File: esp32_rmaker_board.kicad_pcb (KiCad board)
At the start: 2 copper layers, 32 parts, among them Q1 BC817, Q2 BC817, Q3 BC817, Q4 BC817, Q5 BC817, Q6 BC817, U1 ESP32-DevKitC-MCU_Espressif, U10 DHT22, U2 DG142V-5.08-4, U3 DG142V-5.08-4, U4 DG142V-5.08-4, U5 DG142V-5.08-4, U6 LM1117-5.0, U7 DG142V-5.08-4, U9 OPA340NA

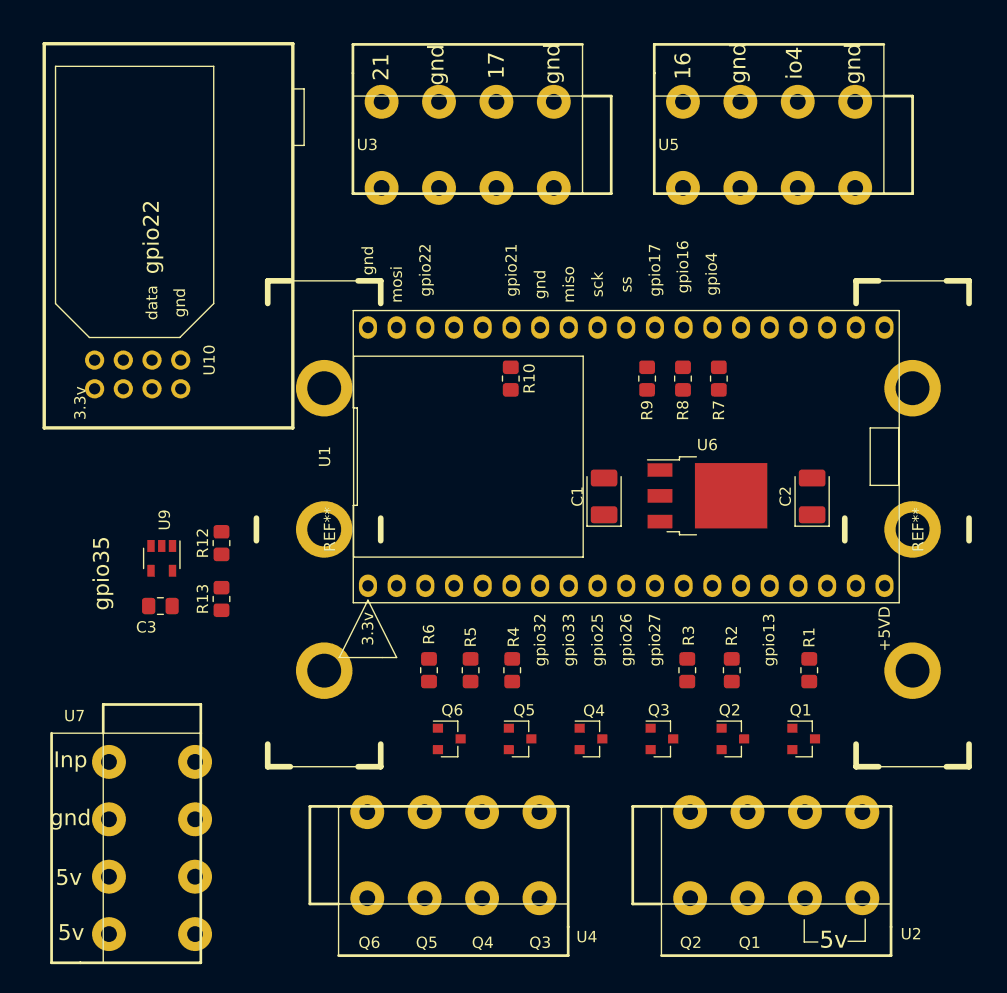
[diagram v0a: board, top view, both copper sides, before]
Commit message: v1.0
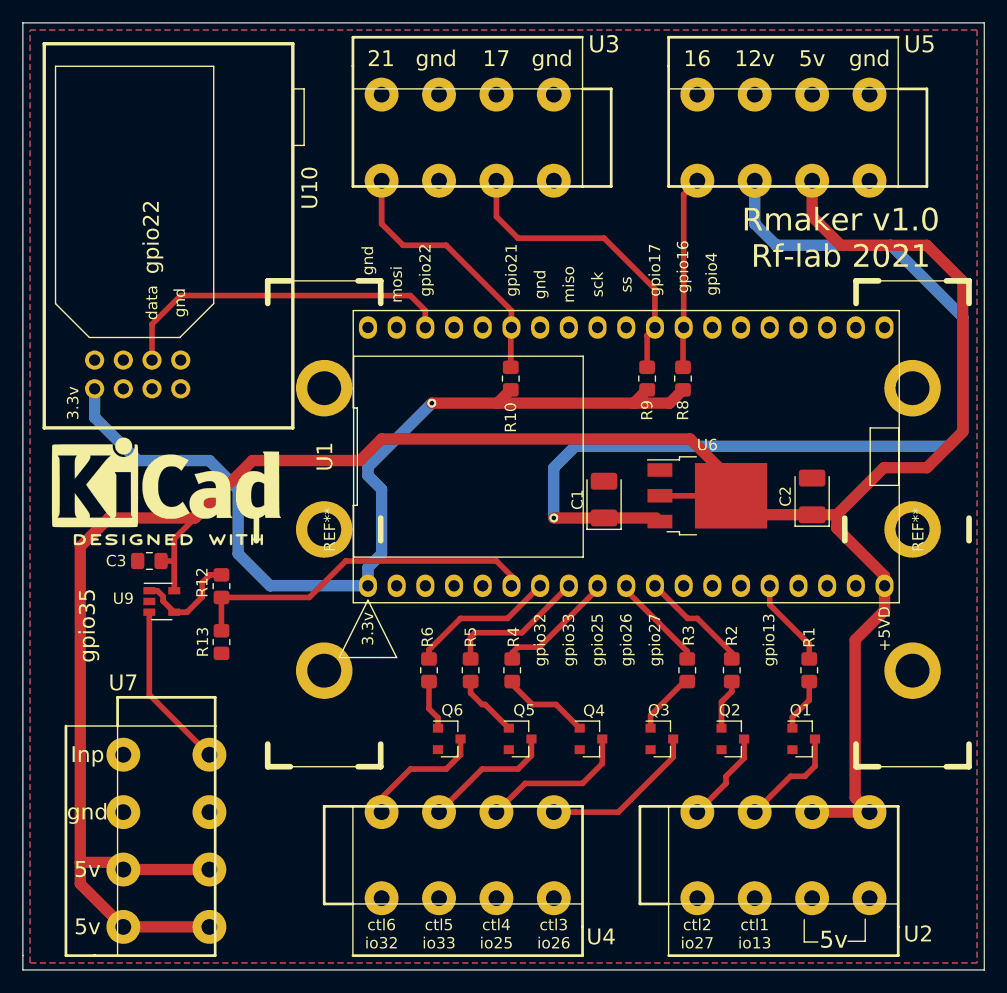
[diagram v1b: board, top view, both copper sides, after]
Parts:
- removed R7: 1k, Resistor_SMD:R_0805_2012Metric_Pad1.20x1.40mm_HandSolder
- added REF**: KiCad-Logo2_8mm_SilkScreen, Symbol:KiCad-Logo2_8mm_SilkScreen, F.Cu at (81.3, 74.9)
- R10, R8, R9: value 1k -> 10k
- moved C3 4.10 mm to (79.8, 81.9)
- moved R12 3.81 mm to (86.2, 84.1)
- moved R13 3.81 mm to (86.2, 89.1)
- moved U9 3.81 mm to (80.9, 85.5), turned to 0 degrees
- moved U7 1.42 mm to (77.5, 99.1)
- moved U5 1.42 mm to (143.5, 40.6)
- moved U4 1.27 mm to (100.3, 111.8)
- moved U2 0.64 mm to (128.3, 111.8)
- moved U3 0.63 mm to (115.6, 40.6)
- moved C1 0.28 mm to (120.0, 76.5)
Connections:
- U1 pad 26: gpio4 -> Net-(U1-Pad26)
- U3 pad 1: Net-(U3-Pad1) -> GND
- U3 pad 3: Net-(U3-Pad3) -> GND
- U5 pad 1: Net-(U5-Pad1) -> GND
- U5 pad 6: GND -> ext_6.5_12v
- U5 pad 7: gpio4 -> 5v
- U7 pad 2: Net-(U7-Pad2) -> GND
- U7 pad 3: Net-(U7-Pad3) -> 5v
- U7 pad 4: Net-(U7-Pad4) -> 5v
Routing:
- net 5v: track 0.00 -> 224.9 mm
- net ext_6.5_12v: track 0.00 -> 87.3 mm, vias 0 -> 1
- net 3v3: track 0.00 -> 81.8 mm, vias 0 -> 1
- net gpio35: track 0.00 -> 31.4 mm
- net gpio22: track 0.00 -> 30.5 mm
- net gpio17: track 0.00 -> 27.1 mm
- net gpio21: track 0.00 -> 23.5 mm
- net gpio16: track 0.00 -> 17.0 mm
- net adcInp: track 0.00 -> 14.8 mm
- net outCtl3: track 0.00 -> 14.2 mm
- net outCtl4: track 0.00 -> 13.3 mm
- net gpio32: track 0.00 -> 13.0 mm
- net gpio33: track 0.00 -> 12.5 mm
- net outCtl5: track 0.00 -> 11.7 mm
- net outCtl6: track 0.00 -> 11.2 mm
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- added copper zone on B.Cu, net GND
- added copper zone on F.Cu, net GND
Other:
- board outline added: 85.1 x 83.8 mm
- net class Default: trace_width 0.25 -> 0.5
- net class highCurrent added: clearance 0.2, trace_width 0.5, via_dia 0.8, via_drill 0.4
- board text added: "12v"
- board text added: "Rmaker v1.0 Rf-lab 2021"
- board text added: "ctl1 io13"
- board text added: "ctl2 io27"
- board text added: "ctl3 io26"
- board text added: "ctl4 io25"
- board text added: "ctl5 io33"
- board text added: "ctl6 io32"
- board text removed: "Q1"
- board text removed: "Q2"
- board text removed: "Q3"
- board text removed: "Q4"
- board text removed: "Q5"
- board text removed: "Q6"
- board text removed: "io4"
